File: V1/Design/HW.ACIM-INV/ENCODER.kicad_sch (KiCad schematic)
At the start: 21 parts, among them J8 ENCODER, Q2 60V/265mA, Q7 60V/265mA, Q8 60V/265mA, Q9 60V/265mA, U9 ISO6740

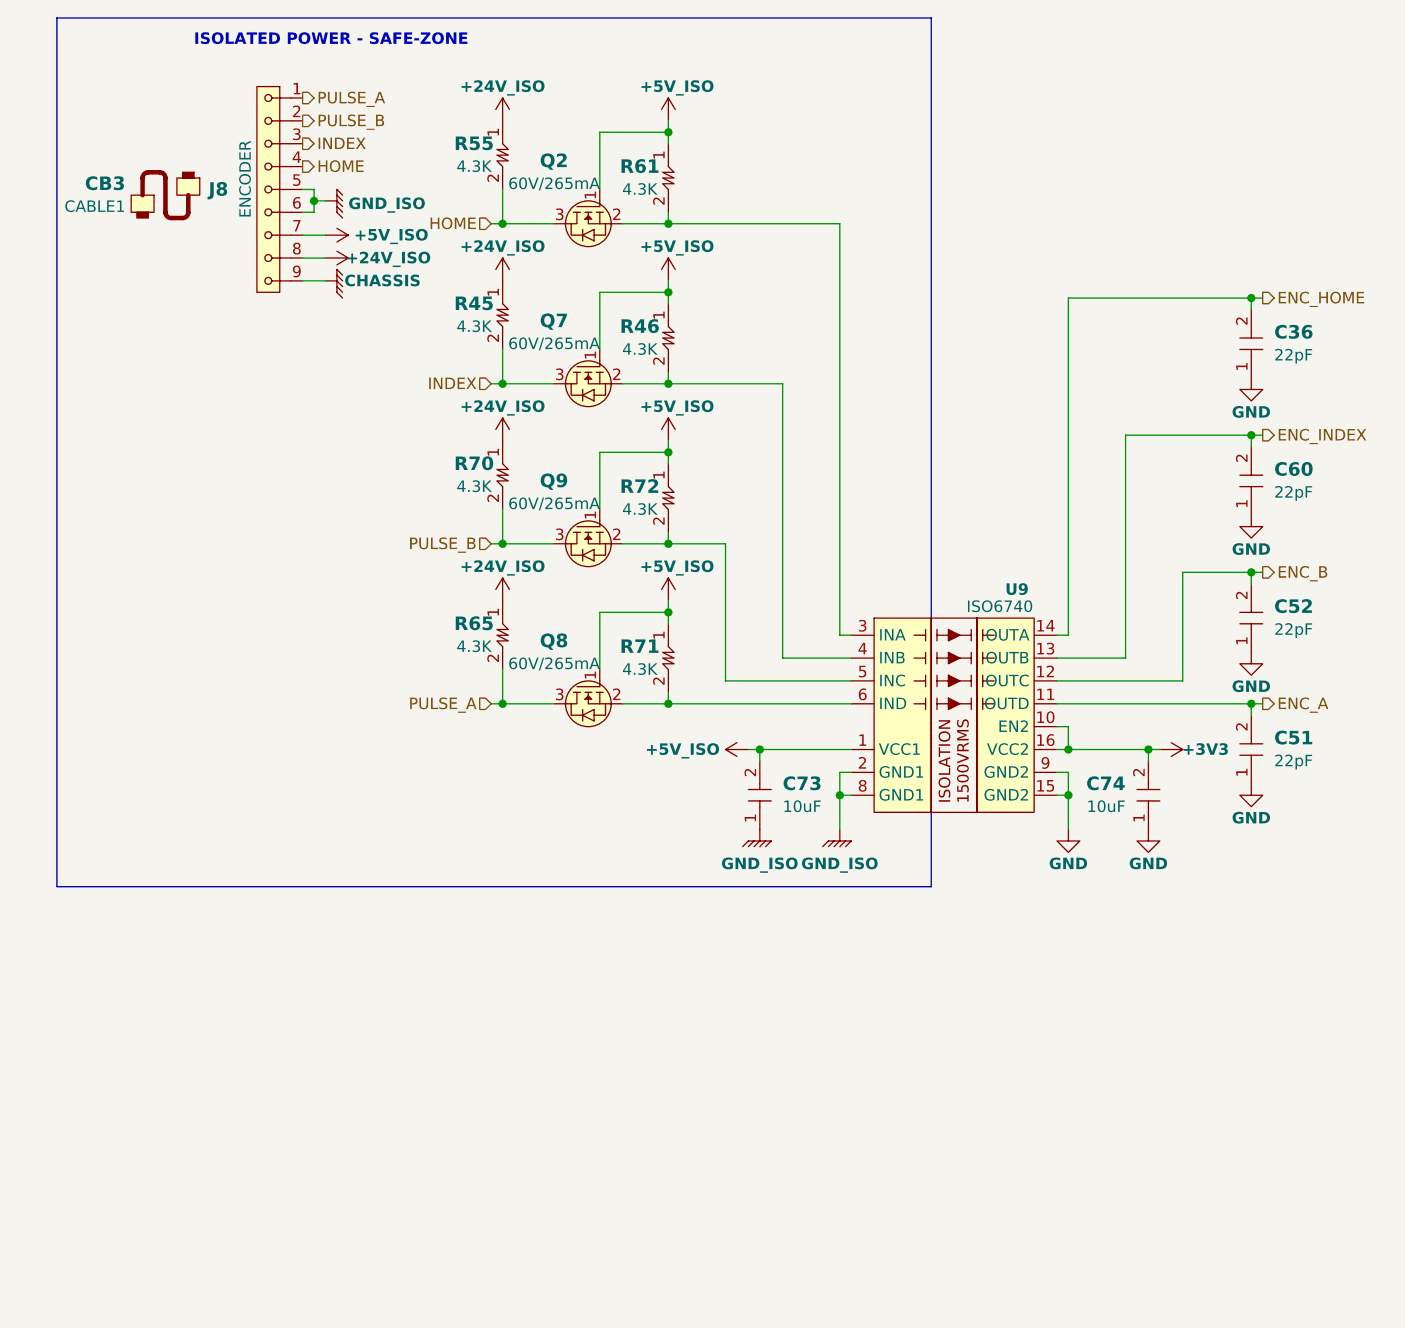
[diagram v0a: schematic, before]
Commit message: V1 schematic update 11
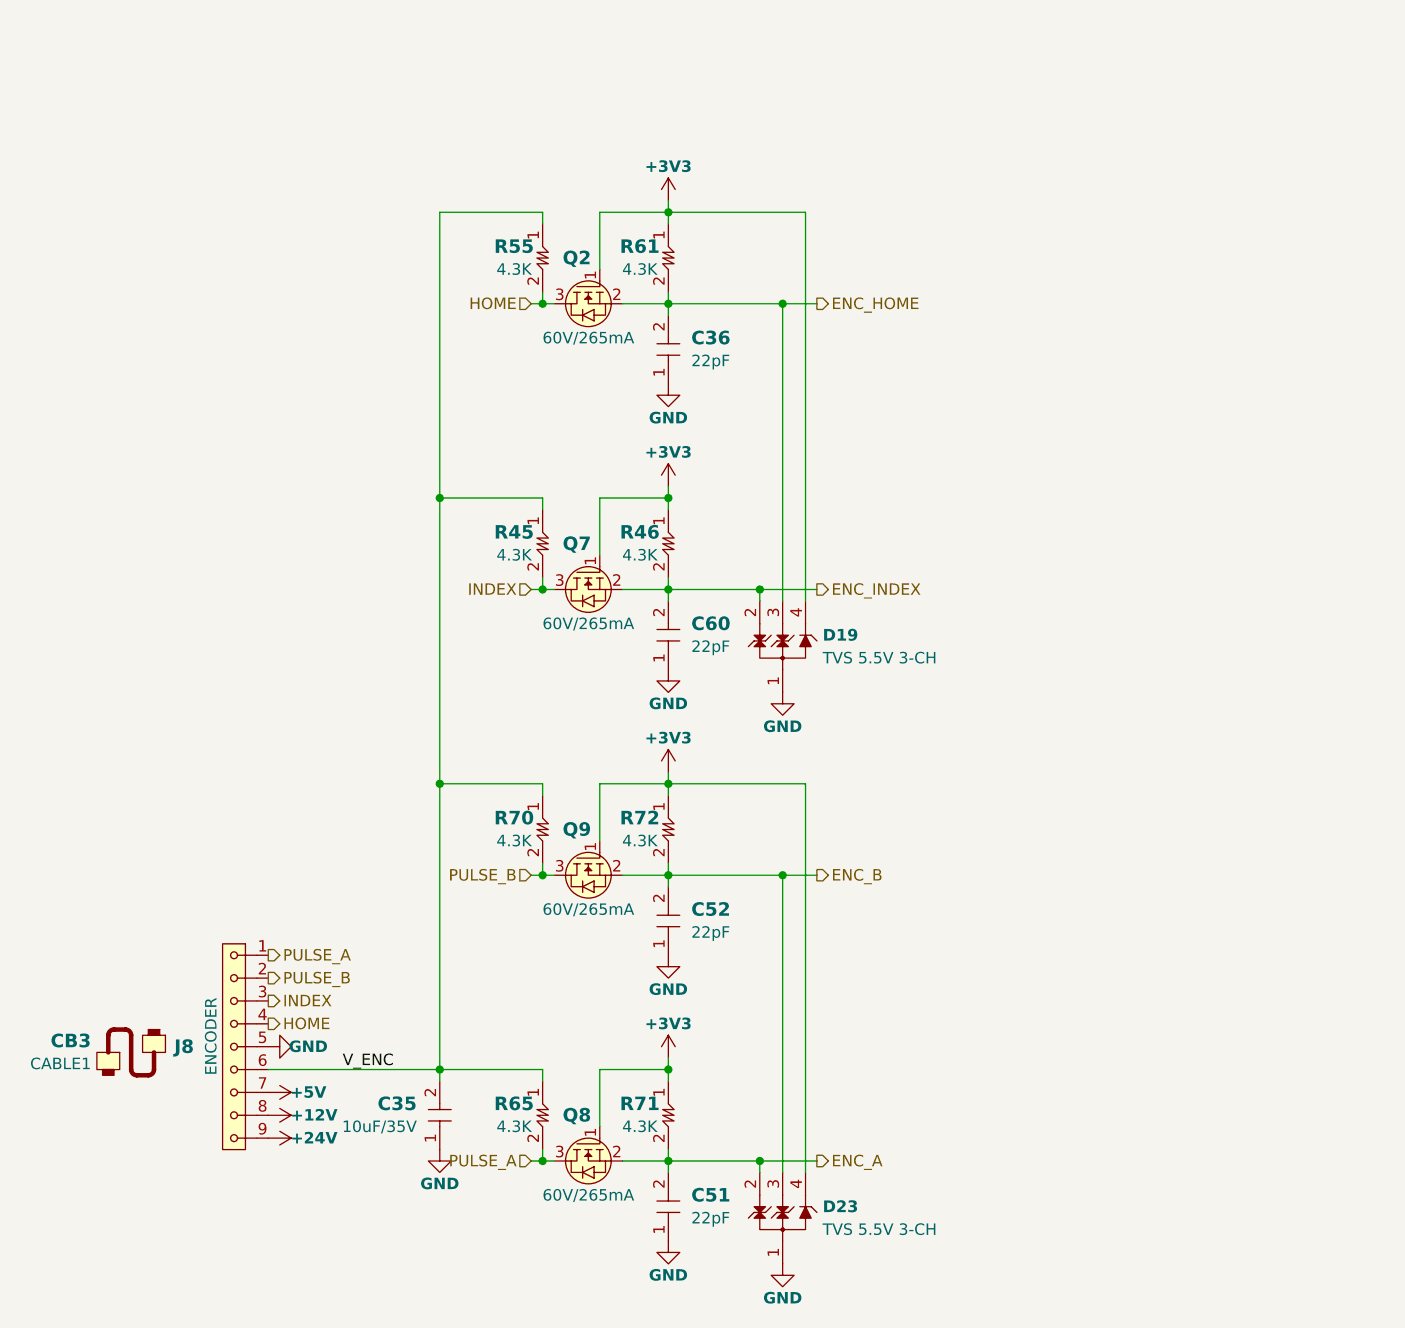
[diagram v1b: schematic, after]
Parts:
- removed C73, C74: 10uF, SAMPI:CAP0603, symbol SAMPI:CERCAP
- removed U9: ISO6740, SAMPI:SOIC16-W, symbol SAMPI:ISO6740
- added C35: 10uF/35V, SAMPI:CAP0603, symbol SAMPI:CERCAP
- added D19, D23: TVS 5.5V 3-CH, SAMPI:SOT143B_NEXT, symbol SAM1:TVS_3CH
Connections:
- net +3V3: now also Q2.1 (G), Q7.1 (G), Q8.1 (G), Q9.1 (G), R46.1, R61.1, R71.1, R72.1, D19.4 (CH3), D23.4 (CH3)
- net ENC_A: now also Q8.2 (S), R71.2, D23.2 (CH1)
- net ENC_B: now also Q9.2 (S), R72.2, D23.3 (CH2)
- net ENC_HOME: now also Q2.2 (S), R61.2, D19.3 (CH2)
- net ENC_INDEX: now also Q7.2 (S), R46.2, D19.2 (CH1)
- net GND: now also J8.5, C35.1, D19.1 (GND), D23.1 (GND)
- net +24V_ISO renamed V_ENC
- net V_ENC: now also J8.6, C35.2; no longer J8.8
- removed net +5V_ISO: J8.7, Q2.1 (G), Q7.1 (G), Q8.1 (G), Q9.1 (G), R46.1, R61.1, R71.1, R72.1
- net CHASSIS renamed +24V
- removed net GND_ISO: J8.5, J8.6
- new net +12V: J8.8
- new net +5V: J8.7
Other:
- note removed: "ISOLATED POWER - SAFE-ZONE"
- moved on the sheet: C36, C51, C52, C60, CB3, J8, Q2, Q7, Q8, Q9, R45, R46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
